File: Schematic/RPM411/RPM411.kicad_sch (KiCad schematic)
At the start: 88 parts, among them J1 02x08_tbd, P1 P_Cap, Q1 tbd (GDS), U1 STM32F100C8Tb8, U2 TS5A9411, U3 TS5A9411, U4 TS5A9411, U5 74LVC3G04, U6 74LVC1G32, U7 TLV70030DDC

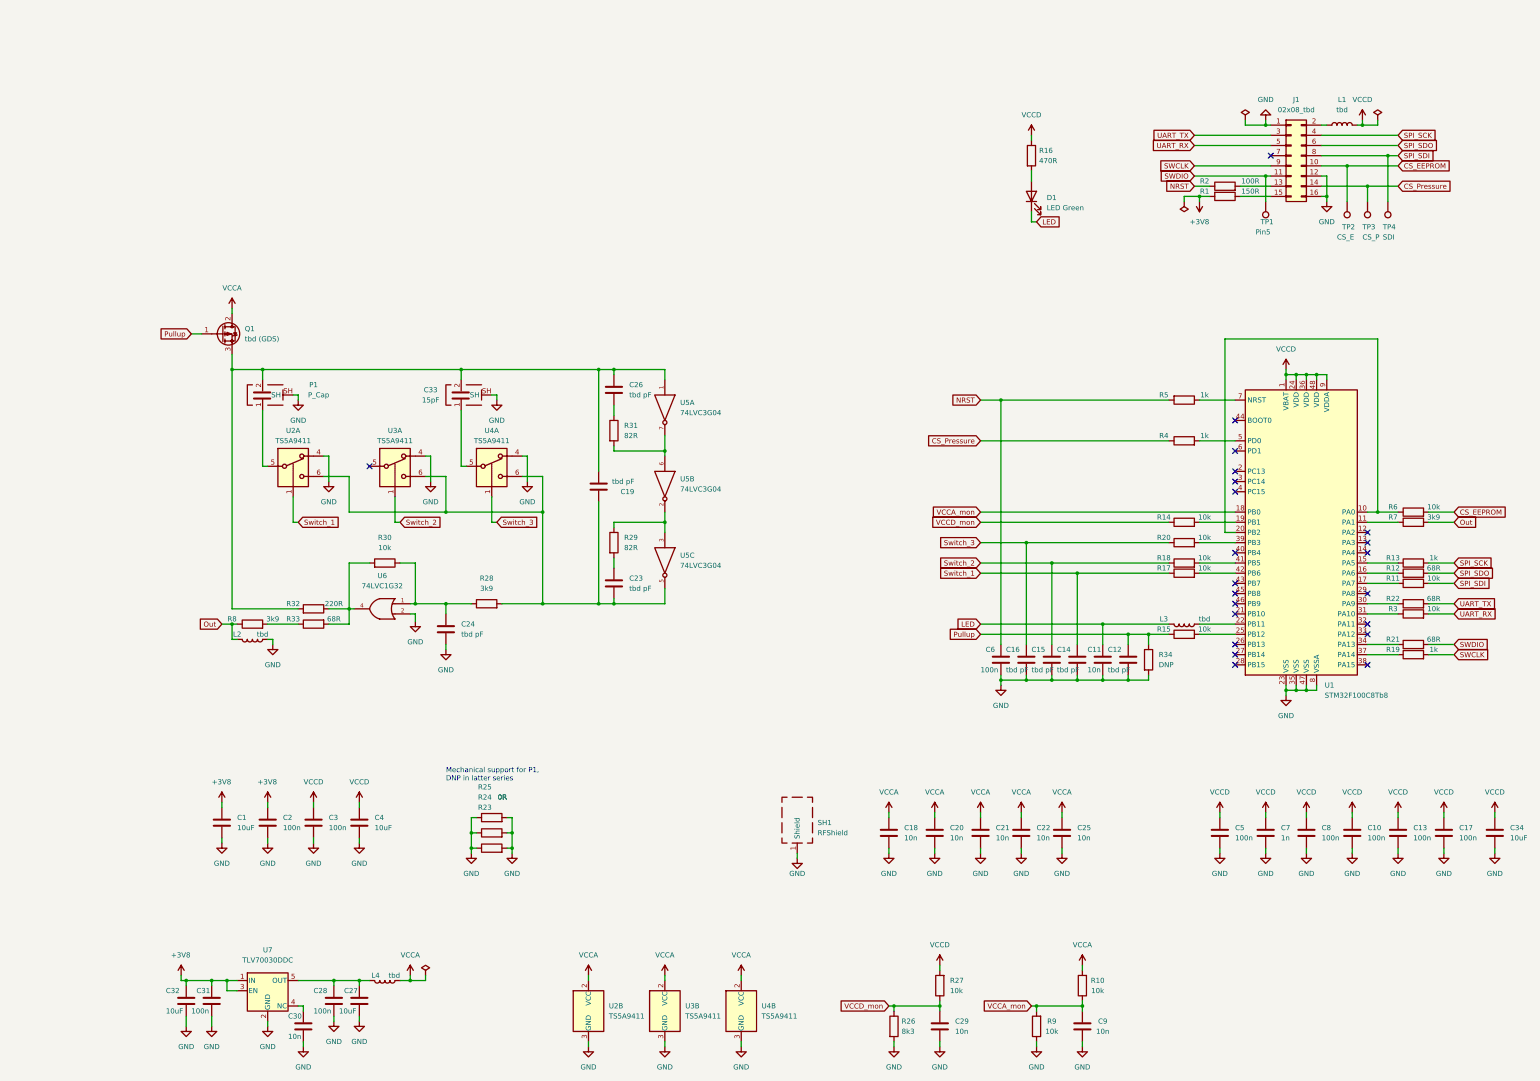
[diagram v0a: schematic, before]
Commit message: sorted schematic
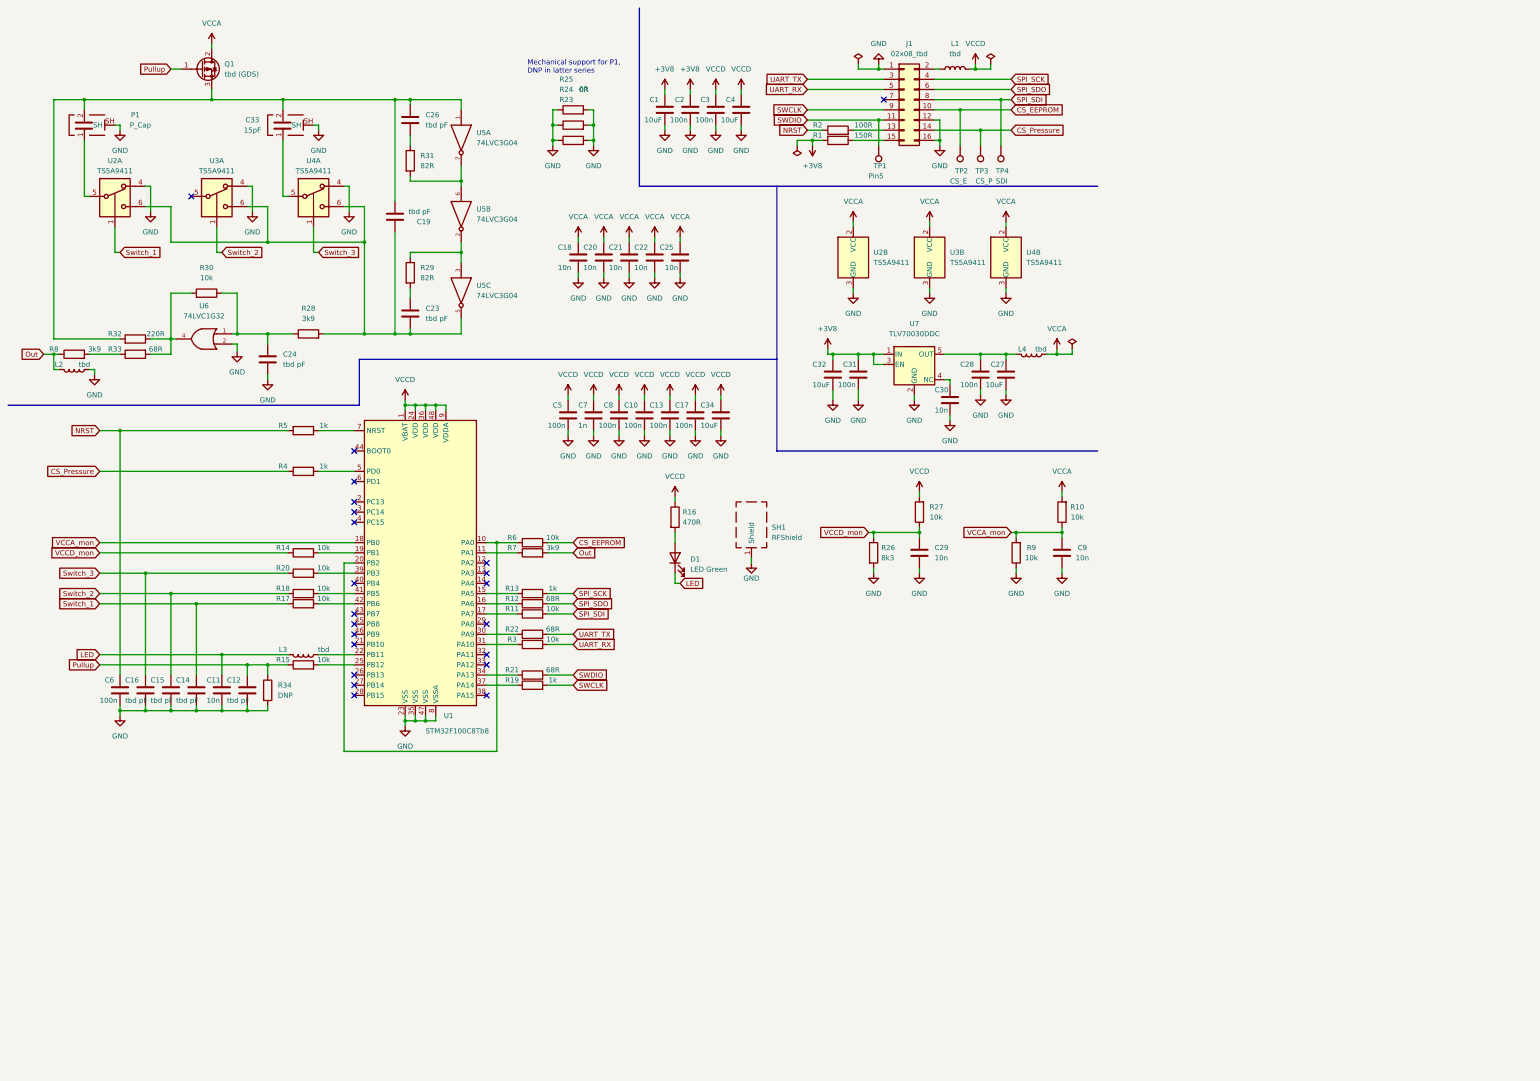
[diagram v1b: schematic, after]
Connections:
- net at U7.4 (NC): now also C30.1
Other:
- company: (none) -> TjarkG
- title: (none) -> RPM411 Pressure Sensor
- moved on the sheet: C1, C10, C11, C12, C13, C14, C15, C16, C17, C18, C19, C2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
